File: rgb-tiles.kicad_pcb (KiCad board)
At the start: 4 copper layers, 99.5 x 99.5 mm, 247 parts, among them J1 SWD, J10 S POWER LINK, J11 W POWER LINK, J2 N / M20-8890645R, J3 E / M20-7910642R, J4 S / M20-7910642R, J5 W / M20-8890645R, J6 USB4110-GF-A, J7 12V INPUT, J8 N POWER LINK, J9 E POWER LINK, Q1 AO3400A, SW1 BOOT, SW2 RESET, U1 RP2040, U10 SN74AHCT1G125DBVR, U11 TPD2E2U06DCKR, U12 TPD2E2U06DCKR, U13 TPD2E2U06DCKR, U14 TPD2E2U06DCKR, U15 TPS26600PWPR, U2 W25Q16JVSSIQ, U3 AP63205WU-7, U4 AP2112K-3.3TRG1, U5 SN74LVC2G125DCUR, U6 SN74LVC2G125DCUR, U7 SN74LVC2G125DCUR, U8 SN74LVC2G125DCUR, U9 USBLC6-2SC6, Y1 ABM8-272-T3 12MHz

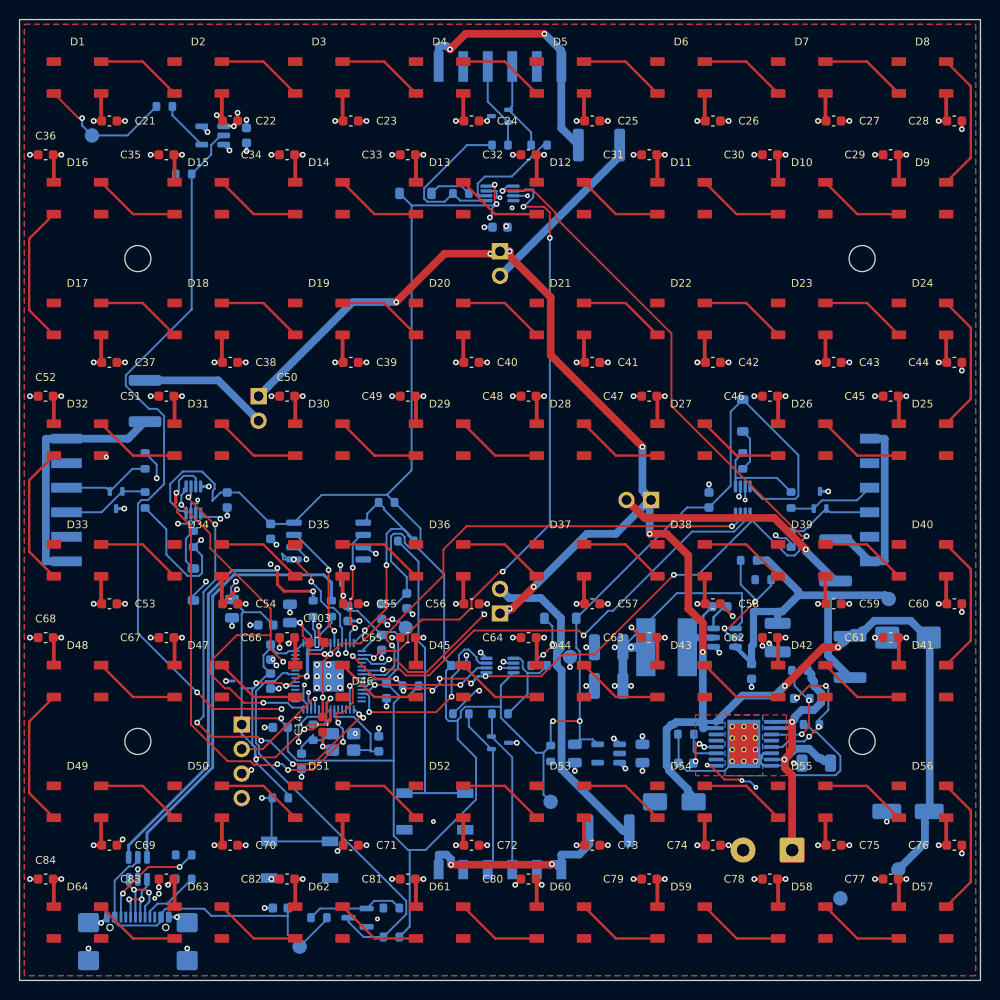
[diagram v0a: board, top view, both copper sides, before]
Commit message: add firmware, controller and manufacturing files
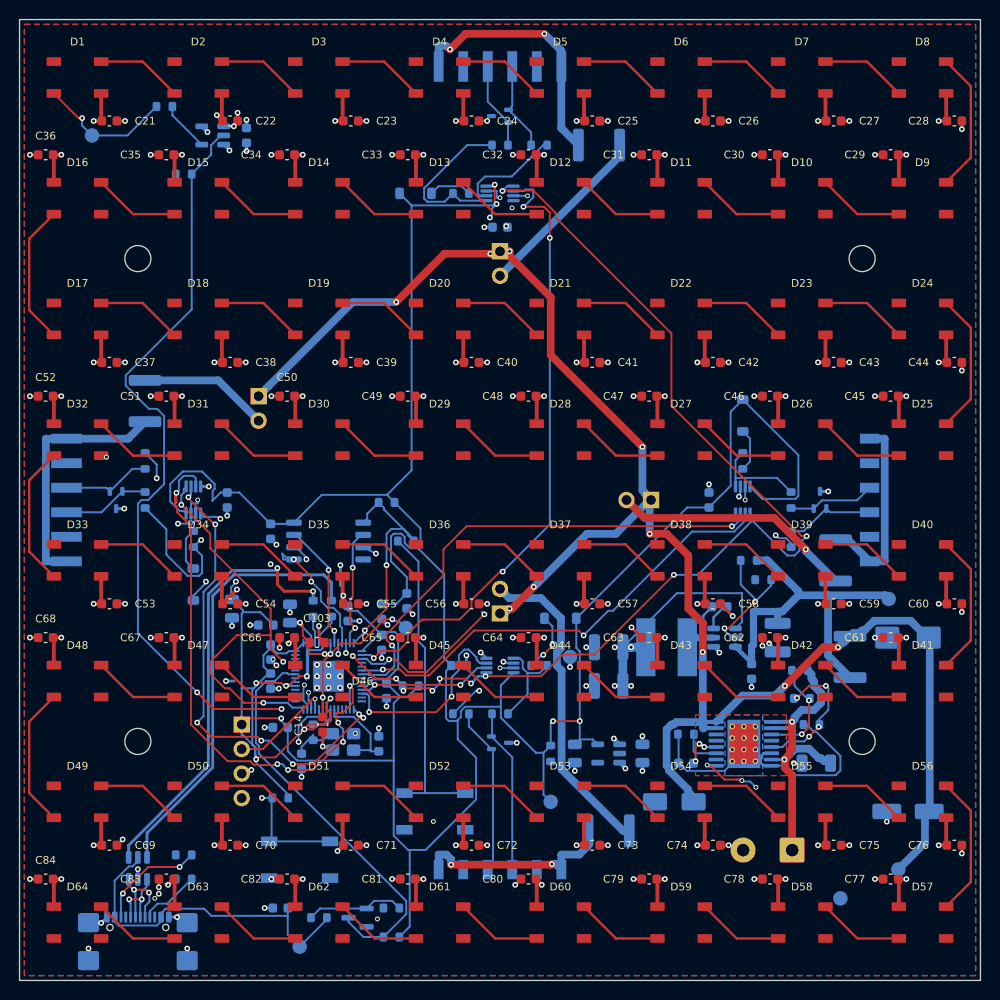
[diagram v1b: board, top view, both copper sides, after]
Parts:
- D70: value SS34 -> B340A
- U11, U12, U13, U14: value TPD2E2U06DCKR -> TPD2E2U06QDCKRQ1
